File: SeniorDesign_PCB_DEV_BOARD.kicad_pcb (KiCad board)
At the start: 4 copper layers, 285.5 x 80.8 mm, 368 parts, among them J1 Conn_01x04_Pin, J10 Conn_01x02_Socket, J11 Conn_01x02_Pin, J12 USB_C_Receptacle_USB2.0_14P, J13 USB_C_Receptacle_USB2.0_14P, J14 IDC_Cable_02x08, J15 Conn_01x02_Pin, J16 Conn_01x04_Pin, J17 Conn_01x04_Pin, J18 Micro_SD_Card, J19 Conn_01x02_Socket, J2 Conn_01x02_Socket, J20 Conn_01x02_Socket, J21 MIC_I2S_CONNECTOR, J22 Conn_01x02_Socket, J23 Conn_01x02_Socket, J24 Conn_01x02_Socket, J3 Conn_01x03_Socket, J4 Conn_01x04_Pin, J5 Conn_01x02_Pin, J6 Conn_01x02_Socket, J7 Conn_01x02_Socket, J8 Conn_01x02_Socket, J9 Barrel_Jack, Q1 NMOS, Q2 NMOS, Q4 AO3400A, Q5 AO3400A, SW2 SW_Push, SW5 SW_Push, SW6 SW_Push, SW7 SW_Push, U1 TMP117xxDRV, U10 INA219AxD, U11 TLV62569ADRL, U12 USBLC6-2P6, U13 USBLC6-2P6, U14 ESP32-C3FH4, U15 TPS60400DBV, U16 TLV172IDCK, U2 RV-3028-C7, U3 STM32G474RETx, U5 MAX98357A, U6 TLV172IDCK, U7 TLV172IDCK, U8 MAX98357A, U9 INA219AxD, Y1 16MHz, Y2 40MHz

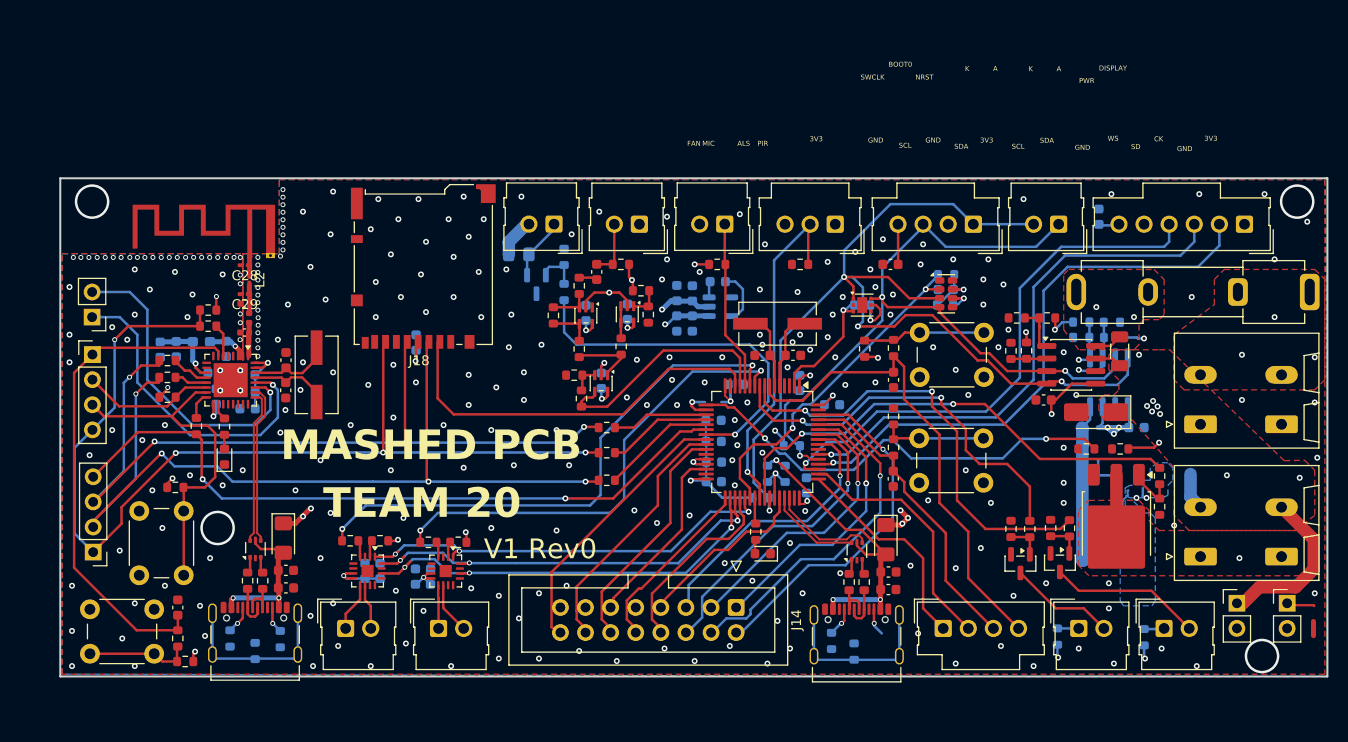
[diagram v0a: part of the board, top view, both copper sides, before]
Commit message: taking a break
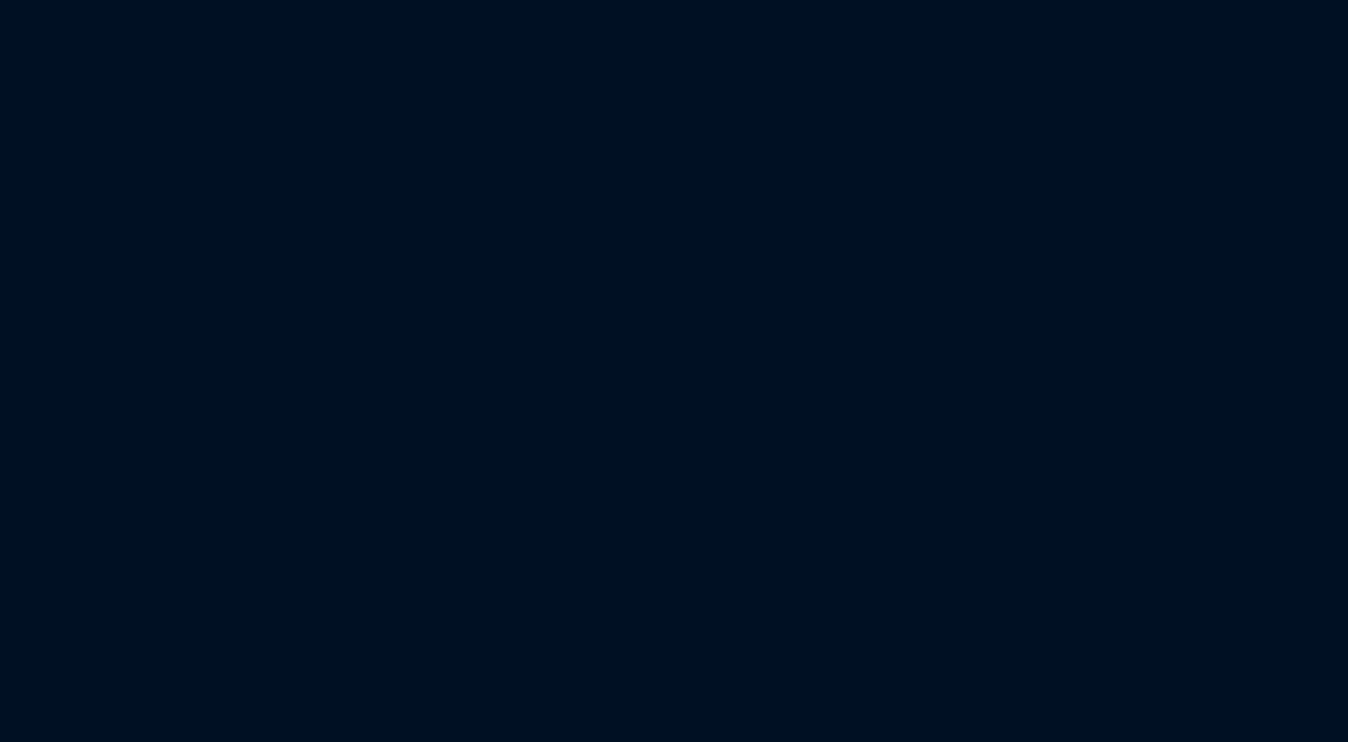
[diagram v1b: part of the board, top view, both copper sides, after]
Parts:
- removed the AE1 at (236.9, 73.7)
- removed the C1 at (283.8, 90.4)
- removed the C10 at (293.2, 96.9)
- removed the C11 at (302.0, 96.3)
- removed the C12 at (250.1, 105.6)
- removed the C13 at (248.6, 105.6)
- removed the C14 at (301.7, 74.6)
- removed the C15 at (272.0, 75.3)
- removed the C16 at (255.2, 106.2)
- removed the C17 at (253.7, 106.2)
- removed the C18 at (317.2, 88.3)
- removed the C19 at (326.6, 91.1)
- removed the C2 at (283.9, 94.6)
- removed the C22 at (301.5, 107.5)
- removed the C23 at (240.6, 107.3)
- removed the C24 at (301.5, 105.7)
- removed the C25 at (240.6, 105.5)
- removed the C26 at (240.6, 87.3)
- removed the C27 at (240.6, 84.3)
- removed the C28 at (236.4, 74.7)
- removed the C29 at (236.4, 77.6)
- removed the C3 at (283.8, 92.5)
- removed the C30 at (236.4, 78.5)
- removed the C31 at (236.4, 81.5)
- removed the C32 at (236.7, 85.8)
- removed the C33 at (234.5, 83.1)
- removed the C34 at (236.7, 87.5)
- removed the C35 at (233.5, 85.6)
- removed the C36 at (229.5, 83.2)
- removed the C37 at (233.5, 88.0)
- removed the C38 at (227.9, 83.2)
- removed the C39 at (236.7, 89.2)
- removed the C4 at (283.9, 96.6)
- removed the C40 at (272.5, 86.3)
- removed the C41 at (253.7, 82.5)
- removed the C42 at (302.0, 86.3)
- removed the C43 at (284.3, 76.3)
- removed the C44 at (270.9, 79.5)
- removed the C45 at (229.6, 109.3)
- removed the C46 at (307.3, 77.1)
- removed the C47 at (281.7, 77.5)
- removed the C48 at (280.1, 77.5)
- removed the C49 at (281.7, 80.6)
- removed the C5 at (295.8, 88.8)
- removed the C50 at (280.1, 80.6)
- removed the C52 at (322.8, 69.8)
- removed the C53 at (275.1, 79.4)
- removed the C6 at (292.5, 86.6)
- removed the C7 at (286.1, 86.7)
- removed the C8 at (291.9, 83.8)
- removed the C9 at (288.8, 83.8)
- removed the D2 at (288.8, 103.8)
- removed the D4 at (322.5, 89.5)
- removed the D6 at (240.3, 102.3)
- removed the D7 at (301.3, 102.4)
- removed the D8 at (264.1, 73.6)
- removed the D9 at (234.4, 94.0)
- removed the F1 at (344.1, 77.4)
- removed the J1 at (310.1, 70.5)
- removed the J10 at (333.1, 104.1)
- removed J11: Conn_01x02_Pin, Connector_PinHeader_2.54mm:PinHeader_1x02_P2.54mm_Vertical
- removed the J12 at (298.3, 112.0)
- removed the J13 at (237.5, 111.8)
- removed the J14 at (286.1, 109.3)
- removed the J15 at (267.7, 70.5)
- removed the J16 at (221.1, 103.7)
- removed the J17 at (221.0, 83.7)
- removed the J18 at (254.5, 74.8)
- removed the J19 at (329.4, 111.4)
- removed the J2 at (285.0, 70.5)
- removed the J20 at (320.8, 111.4)
- removed the J21 at (337.5, 70.5)
- removed J22, J23: Conn_01x02_Socket, Connector_PinHeader_2.54mm:PinHeader_1x02_P2.54mm_Vertical
- removed J24: Conn_01x02_Socket, Connector_Phoenix_SPT:PhoenixContact_SPT_2.5_2-H-5.0_1x02_P5.0mm_Horizontal
- removed the J3 at (296.1, 70.5)
- removed the J4 at (307.1, 111.4)
- removed the J5 at (318.8, 70.5)
- removed the J6 at (276.3, 70.5)
- removed the J7 at (246.6, 111.4)
- removed the J8 at (256.0, 111.4)
- removed the L2 at (236.9, 76.1)
- removed the L3 at (236.8, 80.0)
- removed the L4 at (232.0, 82.4)
- removed the Q1 at (324.6, 100.9)
- removed the Q2 at (265.9, 76.6)
- removed the Q4 at (318.9, 104.8)
- removed the Q5 at (314.9, 104.9)
- removed the R10 at (291.1, 95.8)
- removed the R11 at (288.1, 101.6)
- removed the R12 at (273.0, 96.4)
- removed the R13 at (273.0, 93.6)
- removed the R14 at (273.0, 91.1)
- removed the R17 at (302.0, 89.9)
- removed the R18 at (299.1, 83.1)
- removed the R19 at (302.0, 93.1)
- removed the R2 at (298.9, 78.7)
- removed the R20 at (247.1, 102.5)
- removed the R21 at (274.5, 74.6)
- removed the R22 at (270.2, 76.7)
- removed the R23 at (267.6, 79.7)
- removed the R24 at (276.5, 77.2)
- removed the R25 at (277.2, 79.7)
- removed the R26 at (274.5, 82.9)
- removed the R27 at (270.2, 83.1)
- removed the R28 at (269.7, 85.8)
- removed the R29 at (270.5, 88.1)
- removed the R3 at (284.2, 74.6)
- removed the R30 at (255.0, 102.7)
- removed the R31 at (329.0, 96.0)
- removed the R32 at (329.0, 99.1)
- removed the R33 at (324.9, 83.4)
- removed the R34 at (258.0, 102.7)
- removed the R35 at (250.1, 102.5)
- removed the R36 at (292.6, 74.6)
- removed the R37 at (302.0, 83.0)
- removed the R38 at (325.0, 93.2)
- removed the R39 at (321.5, 93.2)
- removed the R45 at (240.0, 112.5)
- removed the R46 at (295.8, 112.7)
- removed the R47 at (234.9, 112.4)
- removed the R48 at (297.5, 106.7)
- removed the R49 at (299.1, 106.7)
- removed the R5 at (288.6, 98.2)
- removed the R50 at (236.7, 106.6)
- removed the R51 at (238.2, 106.6)
- removed the R52 at (268.7, 77.4)
- removed the R53 at (268.7, 73.8)
- removed the R54 at (234.4, 91.0)
- removed the R55 at (228.6, 84.3)
- removed the R56 at (228.6, 86.0)
- removed the R57 at (232.7, 80.8)
- removed the R58 at (231.5, 90.9)
- removed the R59 at (228.6, 88.0)
- removed the R6 at (291.8, 92.9)
- removed the R60 at (232.7, 79.2)
- removed the R61 at (298.1, 113.8)
- removed the R62 at (237.5, 113.7)
- removed the R68 at (315.5, 83.3)
- removed the R69 at (317.6, 80.0)
- removed the R7 at (307.3, 78.7)
- removed the R70 at (313.9, 83.3)
- removed the R71 at (314.5, 80.0)
- removed the R72 at (324.1, 82.0)
- removed the R73 at (324.1, 80.4)
- removed the R74 at (321.0, 80.4)
- removed the R75 at (321.0, 82.0)
- removed the R76 at (229.6, 112.4)
- removed the R78 at (230.4, 114.8)
- removed the R79 at (229.4, 97.1)
- removed the R8 at (307.4, 75.6)
- removed the R80 at (319.8, 101.3)
- removed the R81 at (317.9, 101.2)
- removed the R82 at (327.4, 112.3)
- removed the R83 at (315.8, 101.3)
- removed the R84 at (313.9, 101.3)
- removed the R85 at (318.6, 112.2)
- removed the R9 at (289.3, 95.8)
- removed the SW2 at (304.6, 92.2)
- removed the SW5 at (304.7, 81.5)
- removed the SW6 at (227.2, 114.0)
- removed the SW7 at (230.2, 99.5)
- removed the U1 at (298.9, 78.7)
- removed the U10 at (323.8, 86.5)
- removed the U12 at (298.3, 103.6)
- removed the U13 at (237.5, 103.4)
- removed the U14 at (235.0, 86.3)
- removed the U15 at (284.5, 78.9)
- removed the U16 at (275.1, 79.6)
- removed the U2 at (307.4, 77.6)
- removed the U3 at (288.8, 92.5)
- removed the U5 at (248.8, 105.6)
- removed the U6 at (270.9, 79.8)
- removed the U7 at (272.5, 86.6)
- removed the U8 at (256.7, 105.6)
- removed the U9 at (320.0, 84.7)
- removed the Y1 at (290.3, 80.6)
- removed the Y2 at (243.7, 85.8)
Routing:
- net 3V3: track 277.3 -> 136.7 mm, vias 73 -> 36
- net /ESP32C3/SPI1_MISO: track 235.1 -> 122.9 mm, vias 8 -> 4
- net 5V: track 206.0 -> 98.9 mm, vias 18 -> 12
- net /Power/I2C3_SCL: track 216.6 -> 110.0 mm, vias 7 -> 3
- net /ESP32C3/SPI1_MOSI: track 197.9 -> 98.2 mm, vias 8 -> 4
- net USB_5V: track 214.7 -> 115.4 mm, vias 13 -> 6
- net /ESP32C3/SPI1_SCLK: track 193.6 -> 102.0 mm, vias 8 -> 4
- net /Power/I2C3_SDA: track 172.4 -> 94.3 mm, vias 5 -> 2
- net /ESP32C3/SPI1_CS_ESP: track 177.2 -> 105.4 mm, vias 4 -> 2
- net /STM32G4/I2S3_CK: track 101.2 -> 43.7 mm, vias 2 -> 1
- net /STM32G4/I2S3_WS: track 97.8 -> 42.7 mm, vias 2 -> 1
- net /Analog/LEFT_SD_MODE: track 110.2 -> 55.1 mm, vias 4 -> 2
- net /STM32G4/I2S3_SD: track 95.3 -> 41.0 mm, vias 2 -> 1
- net /ESP32C3/ESP32_RST: track 101.3 -> 50.6 mm
- net /STM32G4/nRST: track 102.1 -> 52.5 mm
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- removed copper zone on B.Cu, net (none)
- removed copper zone on F.Cu, net /Power/5V_AMPS_1
- removed copper zone on F.Cu, net Net-(J10-Pin_1)
- removed copper zone on F.Cu, net Net-(J24-Pin_2)
- removed copper zone on B.Cu, net USB_5V
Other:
- board size 285.5 x 80.8 mm -> 98.3 x 80.8 mm
- board text removed: "MASHED PCB"
- board text removed: "TEAM 20"
- board text removed: "V1 Rev0"
